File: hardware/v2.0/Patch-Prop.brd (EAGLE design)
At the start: 100 x 80 mm, 51 parts, among them IC1 TPS77033, IC2 XBEE, IC3 MMA8452Q, IC4 ATMEGA168, IC5 MCP1253, IC6 W2RV005RM, U2 MCP73831, X1 USBSMD

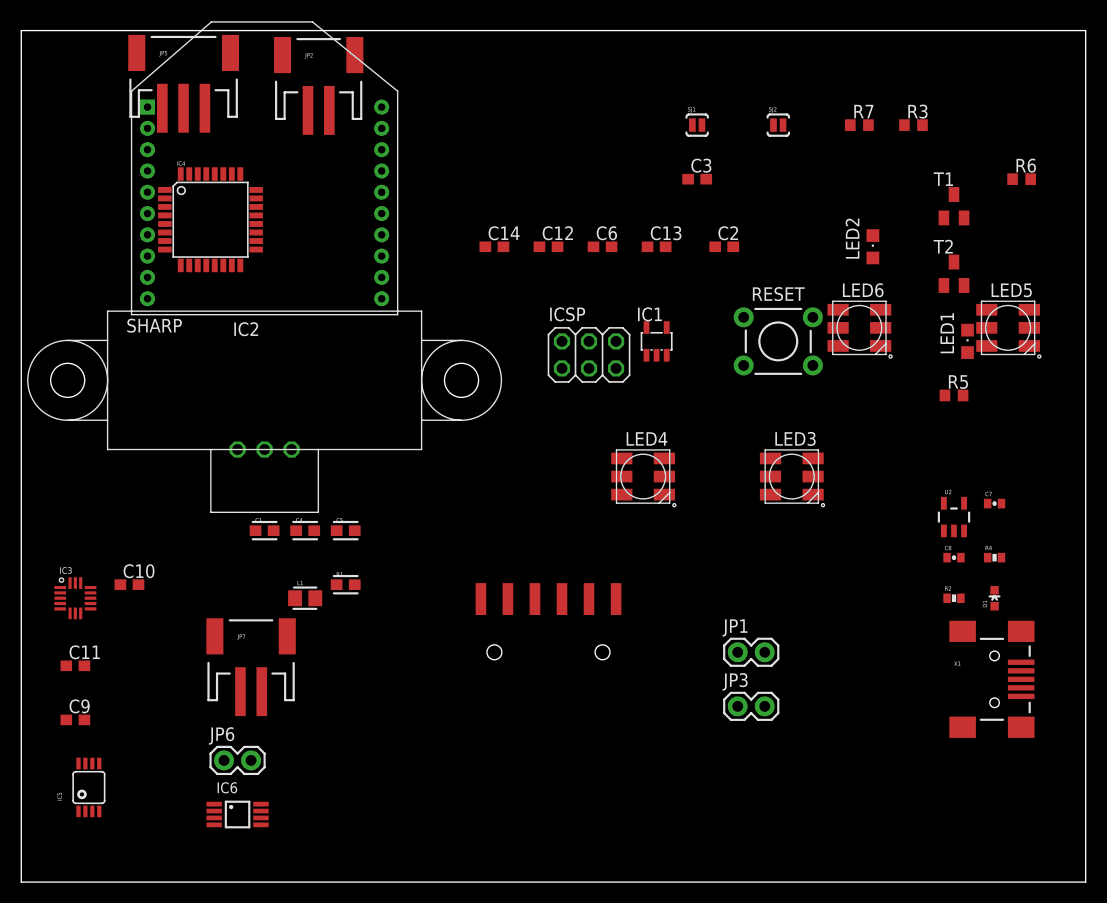
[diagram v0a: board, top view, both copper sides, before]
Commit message: Working on PCB
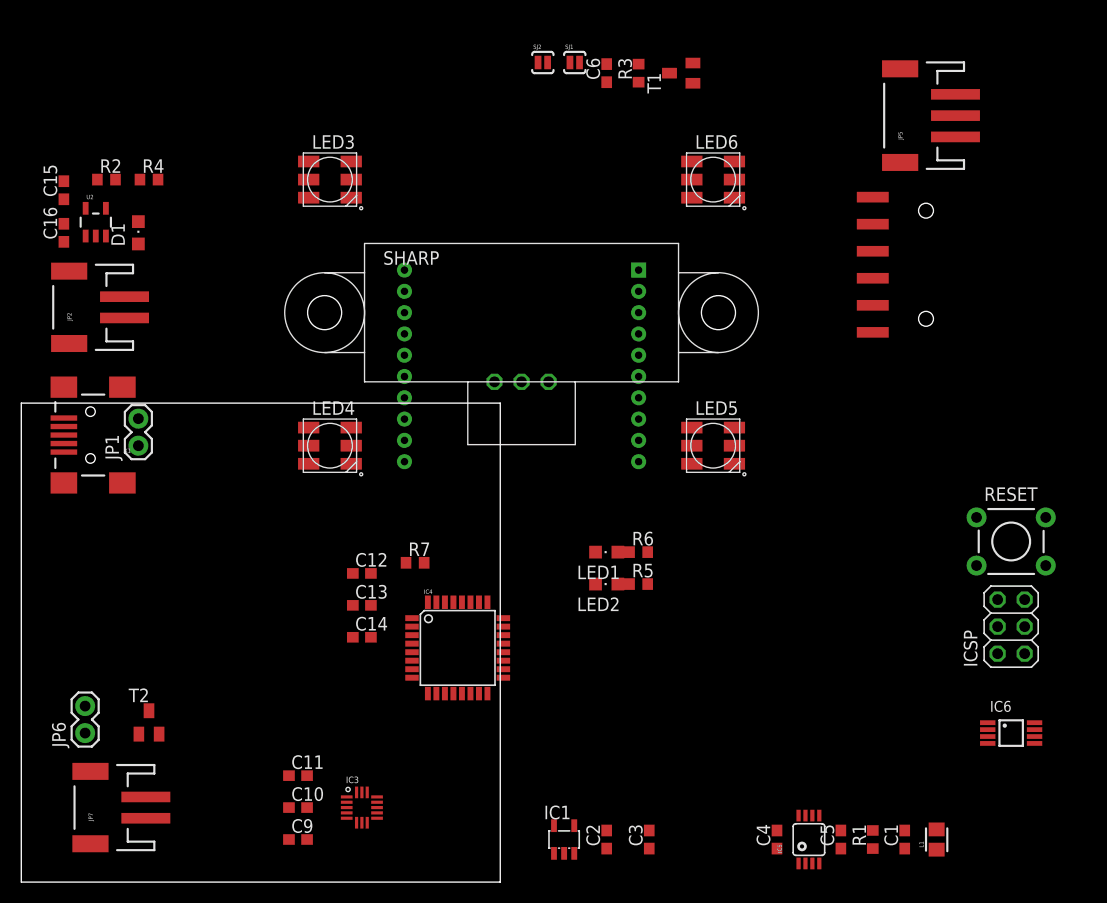
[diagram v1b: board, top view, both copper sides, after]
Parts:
- removed C7, C8: 4.7uF, SparkFun:0402-CAP
- removed JP3: (no value), SparkFun-Connectors:1X02
- added C15, C16: 4.7uF, rcl:C0603
- C1, C4, C5: device CH_passive:0603 -> rcl:C0603
- D1: value Yellow -> (none); device SparkFun:LED-0603 -> led:CHIPLED_0805
- R1: device CH_passive:0603 -> rcl:R0603
- R2: device SparkFun:0402-RES -> rcl:R0603
- R4: value 2K -> 2k; device SparkFun:0402-RES -> rcl:R0603
- moved R2 88.8 mm to (8.00, 66.0)
- moved X1 88.0 mm to (6.50, 42.0), turned to 180 degrees
- moved D1 87.5 mm to (11.0, 61.0)
- moved R4 87.0 mm to (12.0, 66.0)
- moved T2 86.6 mm to (12.0, 15.0)
- moved U2 85.3 mm to (7.00, 62.0)
- moved IC6 73.1 mm to (93.0, 14.0)
- moved JP5 68.0 mm to (83.0, 72.0), turned to 90 degrees
- moved IC5 67.8 mm to (74.0, 4.00)
- moved C1 66.8 mm to (83.0, 4.00), turned to 90 degrees
- moved L1 63.5 mm to (86.0, 4.00), turned to 90 degrees
- moved C3 62.2 mm to (59.0, 4.00), turned to 90 degrees
- moved JP1 59.6 mm to (11.0, 41.0), turned to 90 degrees
- moved R7 58.6 mm to (37.0, 30.0)
- moved C2 56.8 mm to (55.0, 4.00), turned to 90 degrees
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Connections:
- net +3V3: now also C4.1; no longer C4.2
- net GND: now also C15.2, C16.2, C4.2, C5.2; no longer C4.1, C5.1, C7.2, C8.2, JP3.1
- net N$10: now also C5.1, R1.1; no longer C5.2, R1.2
- net PGOOD: now also R1.2; no longer R1.1
- net USB_VIN: now also C16.1; no longer C7.1, JP3.2
- net V+: now also C15.1; no longer C8.1
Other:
- board size 100 x 80 mm -> 45 x 45 mm
